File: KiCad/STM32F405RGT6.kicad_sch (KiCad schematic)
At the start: 32 parts, among them J1 USB_C_Receptacle_USB2.0, J2 USB_C_Receptacle_USB2.0, SW1 SW_SPST, U1 STM32F405RGTx, U2 AT24CS64-SSHM, U3 FT232BM

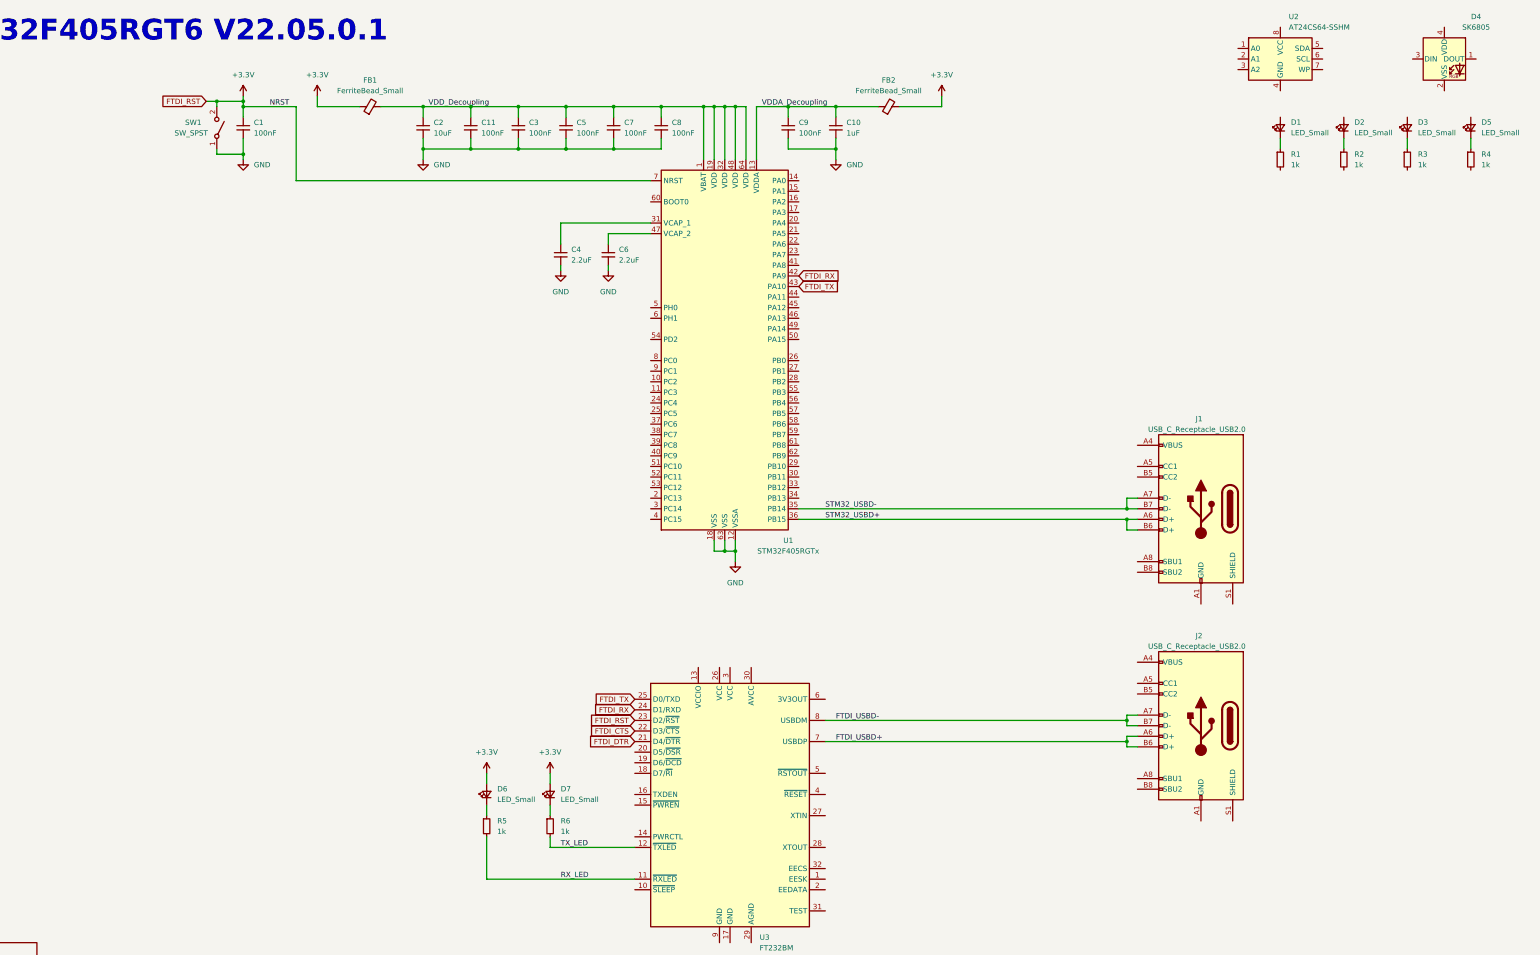
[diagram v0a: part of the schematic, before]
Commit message: Updated Schematic and PCB
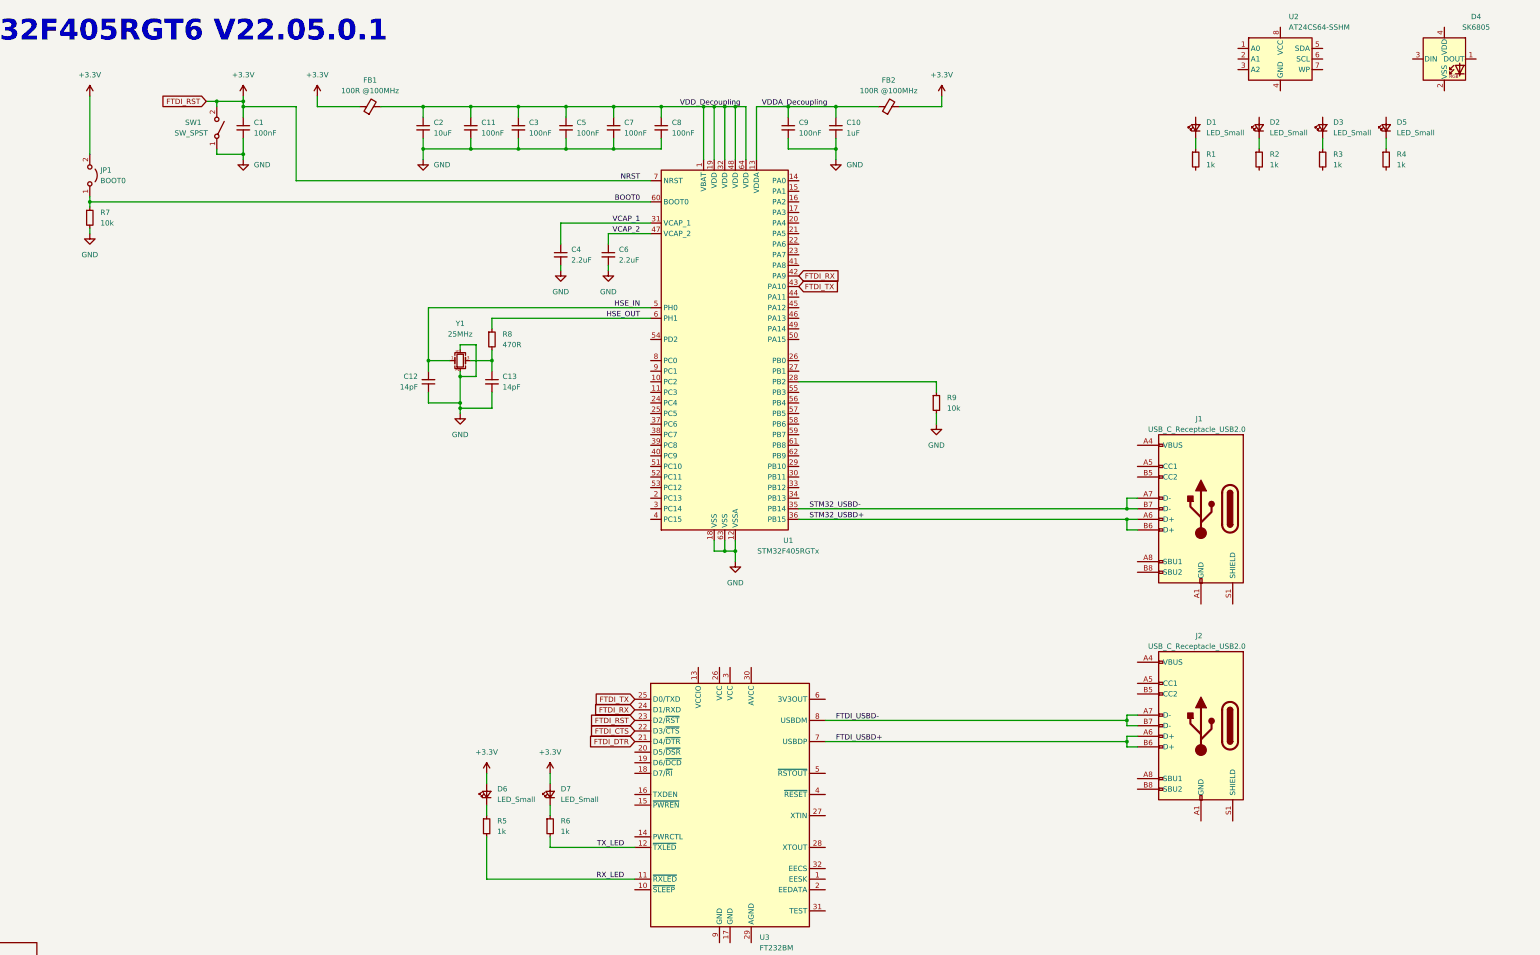
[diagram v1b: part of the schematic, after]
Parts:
- added C12, C13: 14pF, Capacitor_SMD:C_0603_1608Metric, symbol Device:C_Small
- added JP1: BOOT0, Connector_PinHeader_2.54mm:PinHeader_1x02_P2.54mm_Vertical, symbol Jumper:Jumper_2_Open
- added R7, R9: 10k, Resistor_SMD:R_0603_1608Metric, symbol Device:R_Small
- added R8: 470R, Resistor_SMD:R_0603_1608Metric, symbol Device:R_Small
- added Y1: 25MHz, Crystal:Crystal_SMD_3225-4Pin_3.2x2.5mm, symbol Device:Crystal_GND24_Small
- D4: footprint LED_SMD:LED_SK6805_PLCC4_2.4x2.7mm_P1.3mm -> LED_SMD:LED_SK6812_EC15_1.5x1.5mm
- FB1, FB2: value FerriteBead_Small -> 100R @100MHz
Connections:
- net +3V3: now also JP1.2 (B)
- net GND: now also C12.1, C13.2, R7.2, R9.2, Y1.2, Y1.4
- net at U1.28 (PB2): now also R9.1
- net VCAP_1: now reaches C4.1, U1.31 (VCAP_1)
- net VCAP_2: now reaches C6.1, U1.47 (VCAP_2)
- net HSE_IN: now reaches U1.5 (PH0)
- net HSE_IN: now also C12.2, Y1.1
- net HSE_OUT: now reaches U1.6 (PH1)
- net HSE_OUT: now also R8.1
- net BOOT0: now reaches U1.60 (BOOT0)
- net BOOT0: now also JP1.1 (A), R7.1
- new net: C13.1, R8.2, Y1.3
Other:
- moved on the sheet: D1, D2, D3, D5, R1, R2, R3, R4
